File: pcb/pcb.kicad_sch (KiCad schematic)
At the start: 45 parts, among them J1 Conn_01x02_Socket, J2 Conn_01x04_Socket, U1 AP2112K-3.3TRG1, U2 W25Q16JVUXIQ, U3 RP2040, U4 DS4432U+T&amp;R, U5 AD8403ARUZ1-REEL, U6 ADG801BRTZ-REEL7, Y2 Crystal_GND24_Small

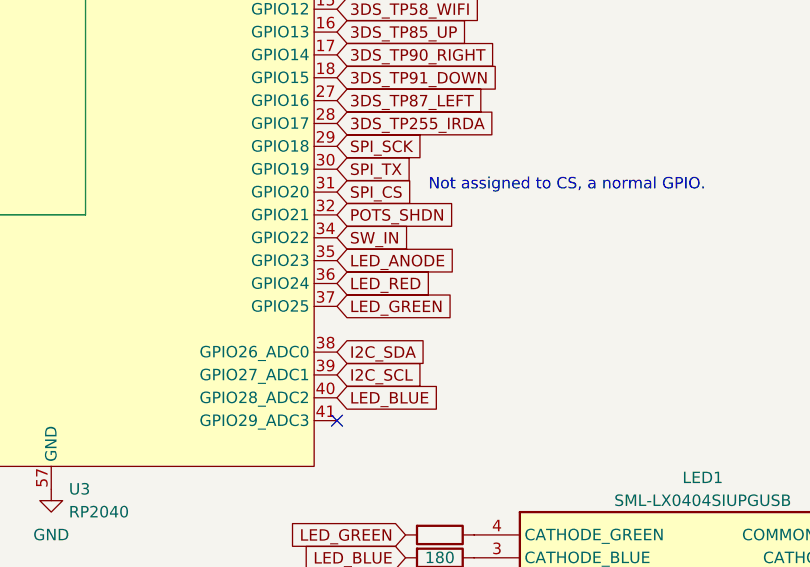
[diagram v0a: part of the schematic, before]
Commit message: Update PCB
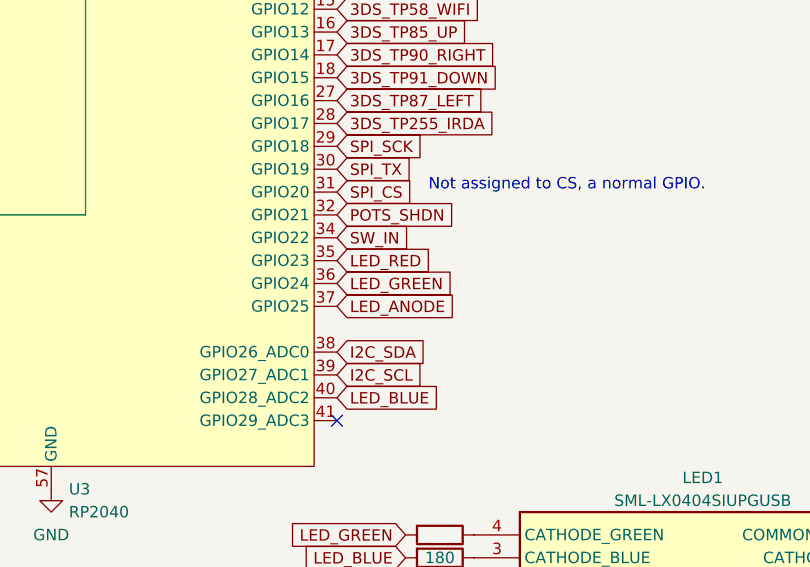
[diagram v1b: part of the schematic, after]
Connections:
- net LED_ANODE: now also U3.37 (GPIO25); no longer U3.35 (GPIO23)
- net LED_GREEN: now also U3.36 (GPIO24); no longer U3.37 (GPIO25)
- net LED_RED: now also U3.35 (GPIO23); no longer U3.36 (GPIO24)
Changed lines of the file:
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@@
-    )
-  )
-  (global_label "LED_RED" (shape input) (at 237.49 127 0) (fields_autoplaced)
-    (effects (font (size 1.27 1.27)) (justify left))
-    (property "Intersheetrefs" "${INTERSHEET_REFS}" (at 248.4995 127 0)
-      (effects (font (size 1.27 1.27)) (justify left) hide)
     )
   )
@@
     )
   )
+  (global_label "LED_GREEN" (shape input) (at 237.49 127 0) (fields_autoplaced)
+    (effects (font (size 1.27 1.27)) (justify left))
+    (property "Intersheetrefs" "${INTERSHEET_REFS}" (at 250.979 127 0)
+      (effects (font (size 1.27 1.27)) (justify left) hide)
+    )
+  )
   (global_label "3DS_TP80_START" (shape input) (at 237.49 88.9 0) (fields_autoplaced)
     (effects (font (size 1.27 1.27)) (justify left))
@@
     )
   )
+  (global_label "LED_ANODE" (shape input) (at 237.49 129.54 0) (fields_autoplaced)
+    (effects (font (size 1.27 1.27)) (justify left))
+    (property "Intersheetrefs" "${INTERSHEET_REFS}" (at 250.9791 129.54 0)
+      (effects (font (size 1.27 1.27)) (justify left) hide)
+    )
+  )
   (global_label "3DS_TP214_Y-" (shape input) (at 134.62 189.23 0) (fields_autoplaced)
     (effects (font (size 1.27 1.27)) (justify left))
@@
     )
   )
+  (global_label "LED_RED" (shape input) (at 237.49 124.46 0) (fields_autoplaced)
+    (effects (font (size 1.27 1.27)) (justify left))
+    (property "Intersheetrefs" "${INTERSHEET_REFS}" (at 248.4995 124.46 0)
+      (effects (font (size 1.27 1.27)) (justify left) hide)
+    )
+  )
   (global_label "SPI_SCK" (shape input) (at 237.49 111.76 0) (fields_autoplaced)
     (effects (font (size 1.27 1.27)) (justify left))
@@
     )
   )
-  (global_label "LED_GREEN" (shape input) (at 237.49 129.54 0) (fields_autoplaced)
-    (effects (font (size 1.27 1.27)) (justify left))
-    (property "Intersheetrefs" "${INTERSHEET_REFS}" (at 250.979 129.54 0)
-      (effects (font (size 1.27 1.27)) (justify left) hide)
-    )
-  )
   (global_label "QSPI_SD1" (shape input) (at 76.2 66.04 180) (fields_autoplaced)
     (effects (font (size 1.27 1.27)) (justify right))
@@
       (effects (font (size 1.27 1.27)) (justify left) hide)
     )
-  )
-  (global_label "LED_ANODE" (shape input) (at 237.49 124.46 0) (fields_autoplaced)
-    (effects (font (size 1.27 1.27)) (justify left))
-    (property "Intersheetrefs" "${INTERSHEET_REFS}" (at 250.9791 124.46 0)
-      (effects (font (size 1.27 1.27)) (justify left) hide)
-    )
